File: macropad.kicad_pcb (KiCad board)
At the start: 2 copper layers, 6 parts, among them J1 OLED_128x32, SW1 SW_Push, SW2 SW_Push, SW3 SW_Push, SW4 RotaryEncoder_Switch, U1 MOUDLE-SEEEDUINO-XIAO

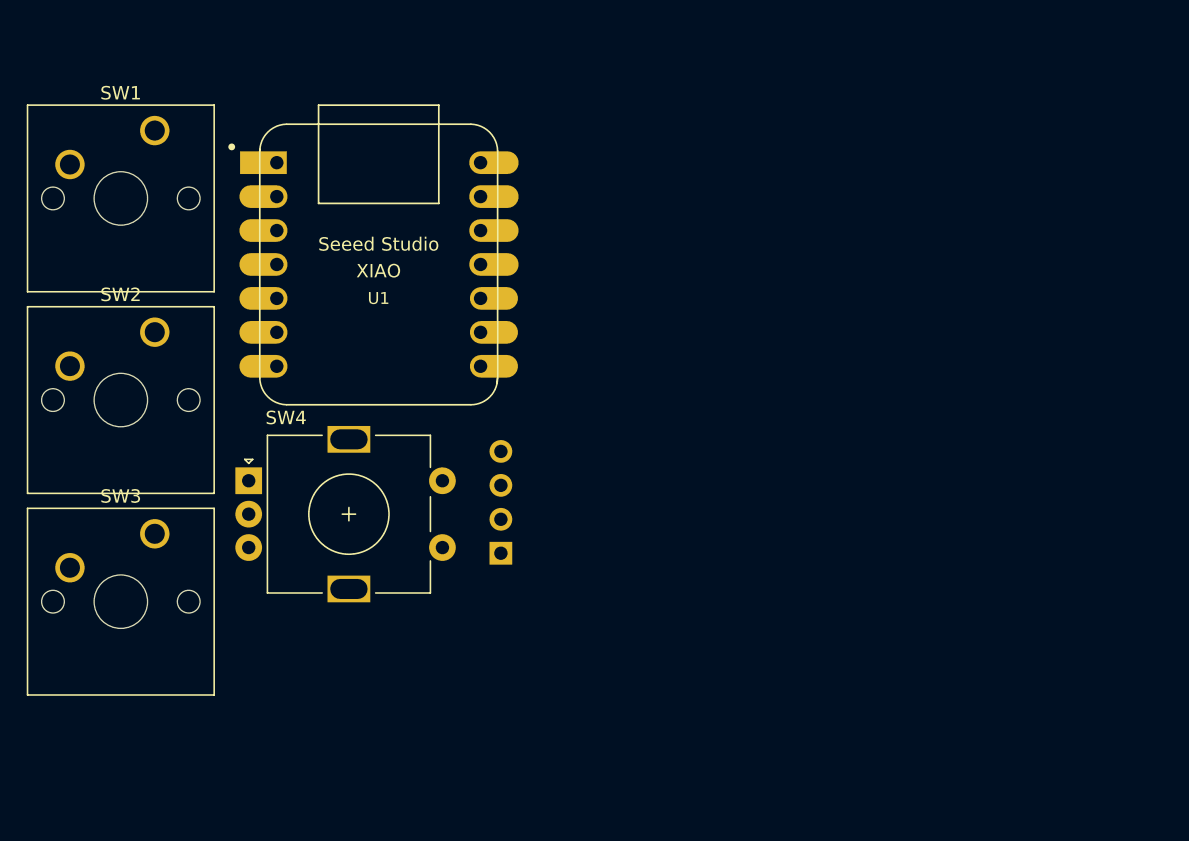
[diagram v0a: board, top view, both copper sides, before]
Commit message: final fixes on pcb + sch files
can't wait to start the model!
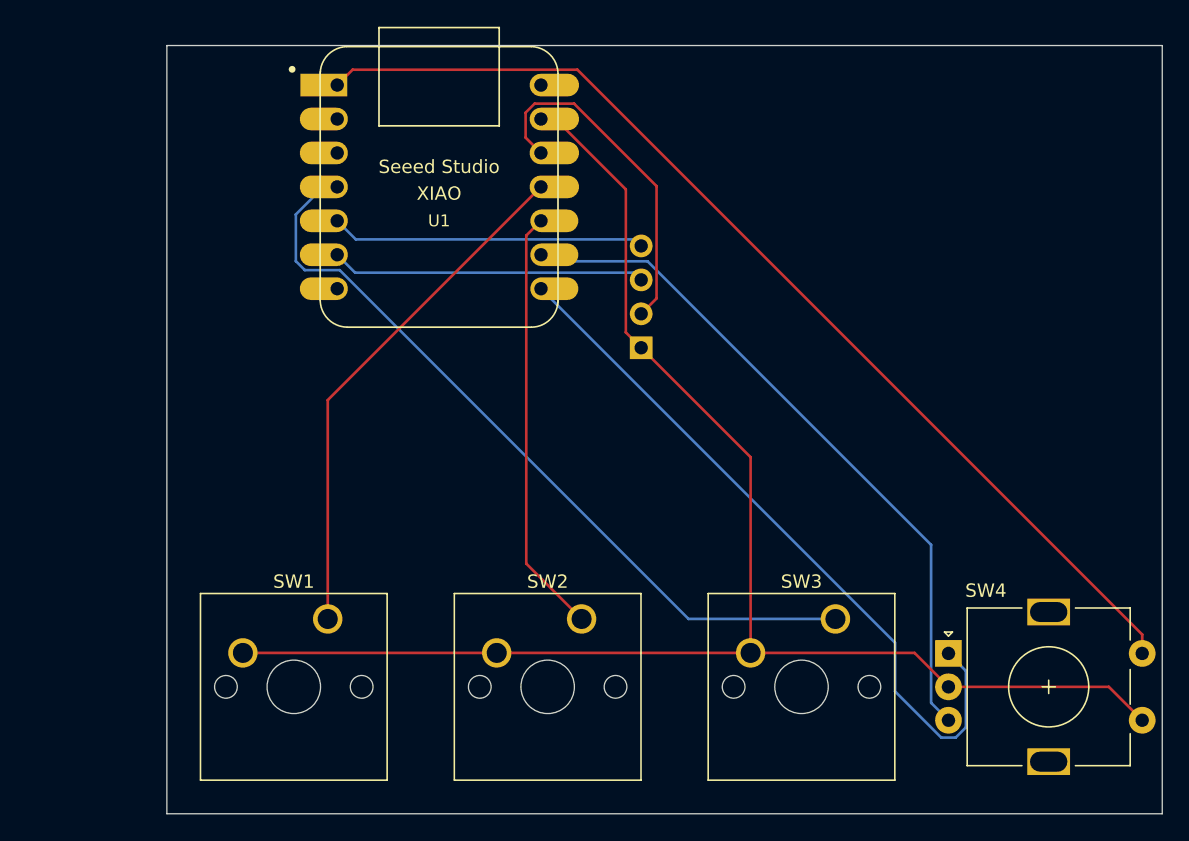
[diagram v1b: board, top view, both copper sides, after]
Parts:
- moved SW4 53.9 mm to (177.0, 120.0)
- moved SW3 51.3 mm to (168.5, 117.4)
- moved SW1 38.8 mm to (130.5, 117.4)
- moved SW2 38.5 mm to (149.5, 117.4)
- moved J1 18.6 mm to (152.4, 87.3)
- moved U1 7.36 mm to (138.9, 85.1)
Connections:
- SW4 pad S1: EC11SWB -> GND
- SW4 pad S2: EC11SWA -> Net-(U1-PA02_A0_D0)
- U1 pad 1: unconnected-(U1-PA02_A0_D0-Pad1) -> Net-(U1-PA02_A0_D0)
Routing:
- net GND: track 0.00 -> 116.5 mm
- net Net-(U1-PA02_A0_D0): track 0.00 -> 79.7 mm
- net Net-(U1-PA11_A3_D3): track 0.00 -> 58.9 mm
- net EC11A: track 0.00 -> 54.2 mm
- net EC11B: track 0.00 -> 51.9 mm
- net Net-(U1-PA6_A10_D10_MOSI): track 0.00 -> 39.0 mm
- net Net-(U1-PA5_A9_D9_MISO): track 0.00 -> 32.0 mm
- net +3.3V: track 0.00 -> 26.2 mm
- net Net-(J1-SCL): track 0.00 -> 23.5 mm
- net Net-(J1-SDA): track 0.00 -> 23.5 mm
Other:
- board outline added: 74.5 x 57.5 mm
